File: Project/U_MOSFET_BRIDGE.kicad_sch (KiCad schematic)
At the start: 14 parts, among them Q301 DMT68M8LFV-7, Q302 DMT68M8LFV-7

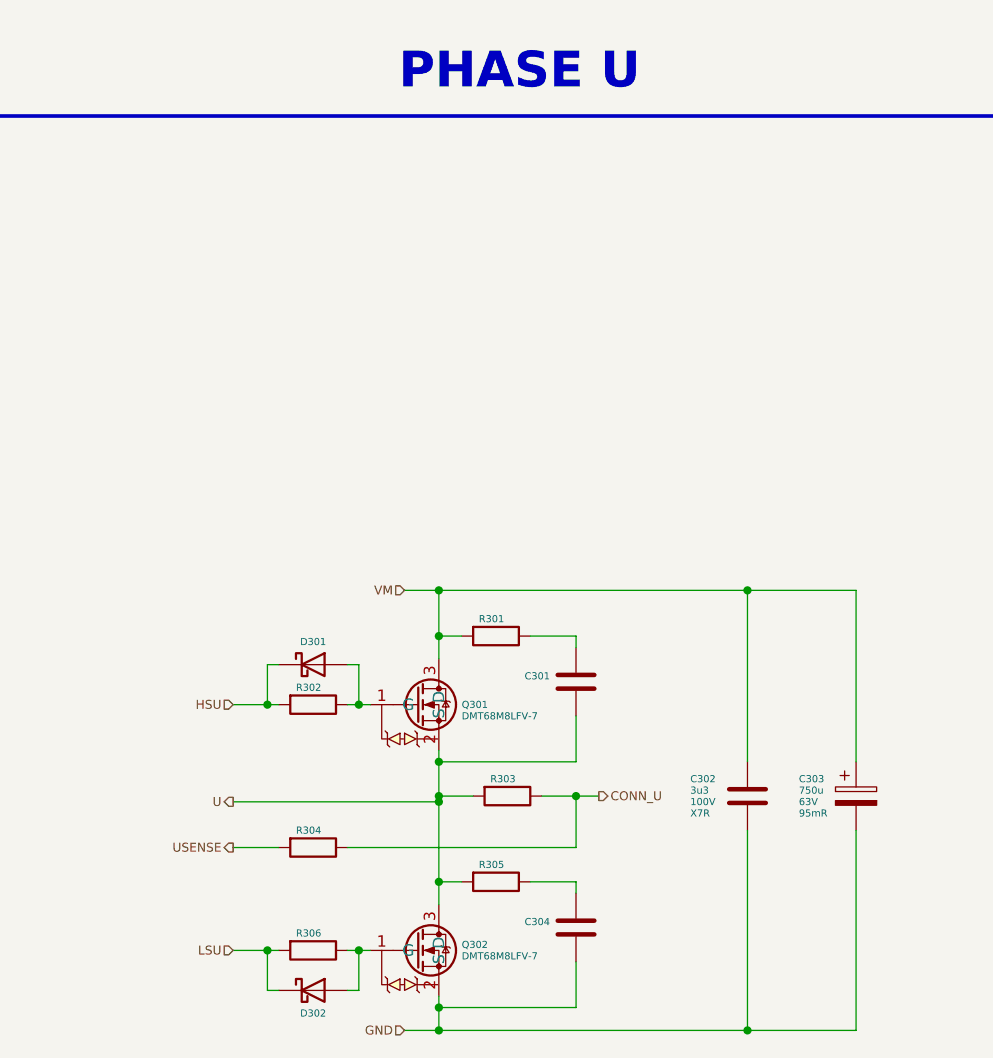
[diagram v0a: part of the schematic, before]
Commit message: Cleanup ED A1 version
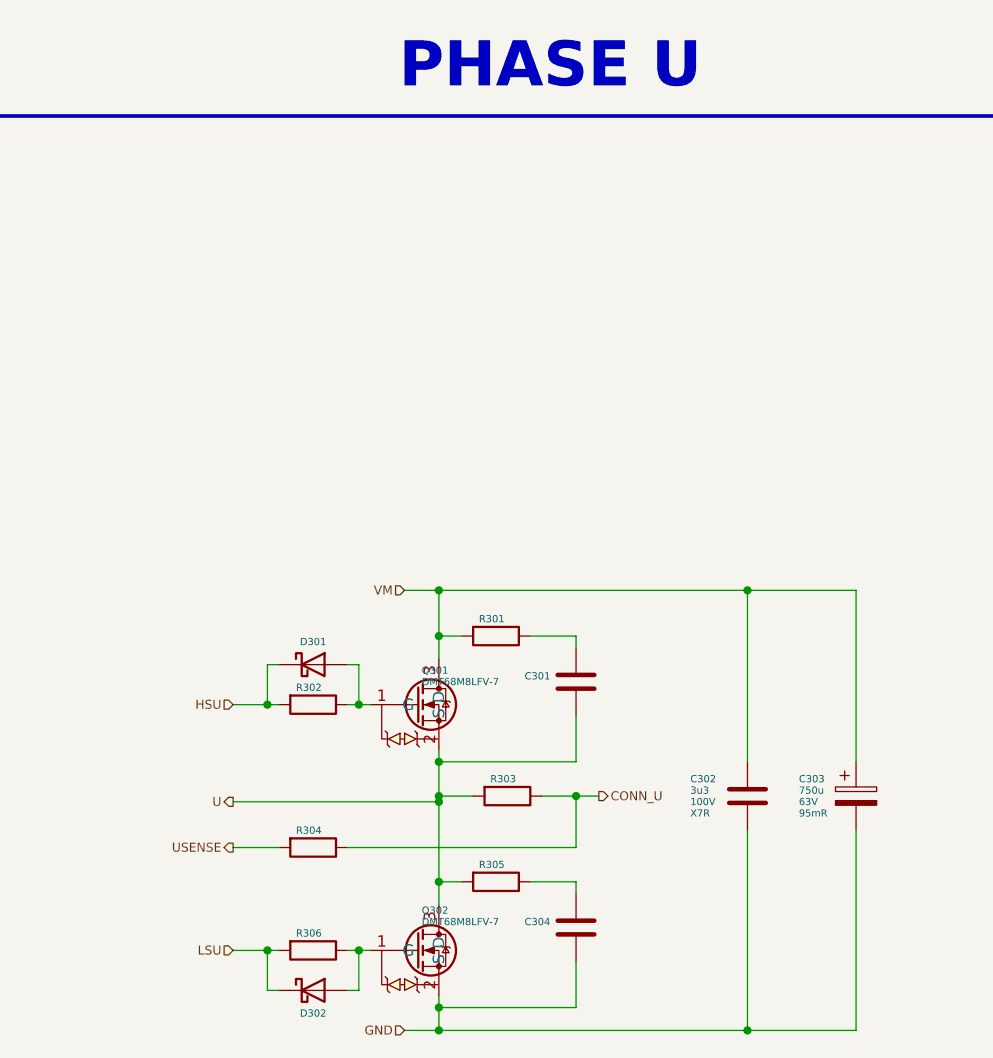
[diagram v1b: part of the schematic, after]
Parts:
- C303: symbol Device:CP -> Device:C_Polarized
- Q301, Q302: symbol eval_board_tmc6200-ta:DMT68M8LFV-7 -> QP_LIBRARY:DMT68M8LFV-7
